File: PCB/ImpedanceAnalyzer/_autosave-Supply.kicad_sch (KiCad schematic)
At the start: 63 parts, among them U18 LM7812_TO220, U19 LM7912_TO220, U20 LM7806_TO220, U21 LT1086-3.3, U22 LM7805_TO220, U23 LM7905_TO220, U24 LM7906_TO220, U28 LD1117S25TR_SOT223

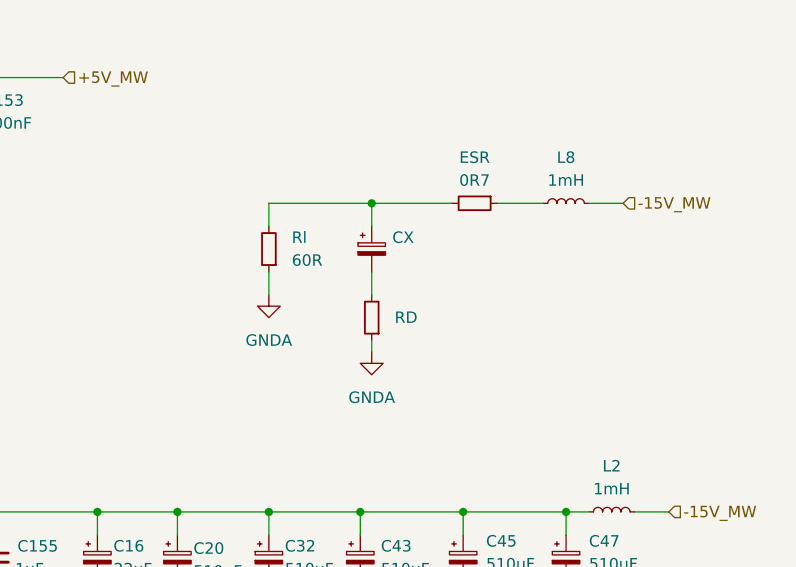
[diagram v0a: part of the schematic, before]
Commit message: docu doneski
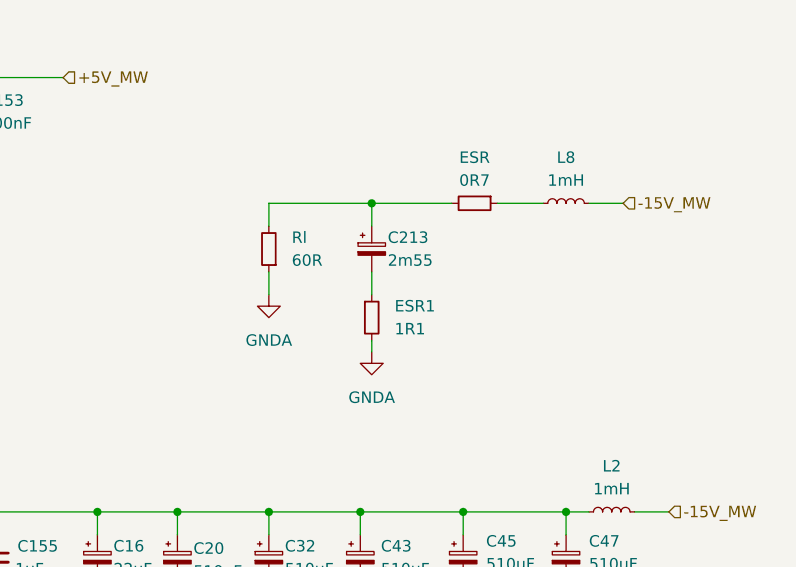
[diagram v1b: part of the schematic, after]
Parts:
- removed CX: CX, Capacitor_THT:CP_Radial_D10.0mm_P5.00mm, symbol Device:C_Polarized_Small
- removed R35: RD, Resistor_THT:R_Axial_DIN0207_L6.3mm_D2.5mm_P10.16mm_Horizontal, symbol Device:R_Small
- added C213: 2m55, Capacitor_THT:CP_Radial_D10.0mm_P5.00mm, symbol Device:C_Polarized_Small
- added ESR1: 1R1, Resistor_THT:R_Axial_DIN0207_L6.3mm_D2.5mm_P10.16mm_Horizontal, symbol Device:R_Small
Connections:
- net GNDA: now also ESR1.2
- net at ESR.2, Rl.2: now also C213.1
- new net: C213.2, ESR1.1
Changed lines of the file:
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@@
 	)
 	(symbol
+		(lib_id "Device:R_Small")
+		(at 228.6 104.14 0)
+		(unit 1)
+		(exclude_from_sim no)
+		(in_bom yes)
+		(on_board yes)
+		(dnp no)
+		(fields_autoplaced yes)
+		(property "Reference" "ESR1"
+			(at 231.14 102.8699 0)
+			(effects
+				(font
+					(size 1.27 1.27)
+				)
+				(justify left)
+			)
+		)
+		(property "Value" "1R1"
+			(at 231.14 105.4099 0)
+			(effects
+				(font
+					(size 1.27 1.27)
+				)
+				(justify left)
+			)
+		)
+		(property "Footprint" "Resistor_THT:R_Axial_DIN0207_L6.3mm_D2.5mm_P10.16mm_Horizontal"
+			(at 228.6 104.14 0)
+			(effects
+				(font
+					(size 1.27 1.27)
+				)
+				(hide yes)
+			)
+		)
+		(property "Datasheet" "~"
+			(at 228.6 104.14 0)
+			(effects
+				(font
+					(size 1.27 1.27)
+				)
+				(hide yes)
+			)
+		)
+		(property "Description" "Resistor, small symbol"
+			(at 228.6 104.14 0)
+			(effects
+				(font
+					(size 1.27 1.27)
+				)
+				(hide yes)
+			)
+		)
+		(pin "2"
+		)
+		(pin "1"
+		)
+		(instances
+			(project "ImpedanceAnalyzer"
+				(path "/08568624-f051-402a-adf3-1b03c2a769ee/bbce87d8-2d6b-4ada-9e87-44e06d8f0f46"
+					(reference "ESR1")
+					(unit 1)
+				)
+			)
+		)
+	)
+	(symbol
 		(lib_id "Device:LED_Small")
 		(at 35.56 160.02 270)
@@
 	(symbol
 		(lib_id "Device:C_Polarized_Small")
+		(at 228.6 96.52 0)
+		(unit 1)
+		(exclude_from_sim no)
+		(in_bom yes)
+		(on_board yes)
+		(dnp no)
+		(property "Reference" "C213"
+			(at 230.378 95.25 0)
+			(effects
+				(font
+					(size 1.27 1.27)
+				)
+				(justify left)
+			)
+		)
+		(property "Value" "2m55"
+			(at 230.378 97.79 0)
+			(effects
+				(font
+					(size 1.27 1.27)
+				)
+				(justify left)
+			)
+		)
+		(property "Footprint" "Capacitor_THT:CP_Radial_D10.0mm_P5.00mm"
+			(at 228.6 96.52 0)
+			(effects
+				(font
+					(size 1.27 1.27)
+				)
+				(hide yes)
+			)
+		)
+		(property "Datasheet" "~"
+			(at 228.6 96.52 0)
+			(effects
+				(font
+					(size 1.27 1.27)
+				)
+				(hide yes)
+			)
+		)
+		(property "Description" "Polarized capacitor, small symbol"
+			(at 228.6 96.52 0)
+			(effects
+				(font
+					(size 1.27 1.27)
+				)
+				(hide yes)
+			)
+		)
+		(pin "1"
+		)
+		(pin "2"
+		)
+		(instances
+			(project "ImpedanceAnalyzer"
+				(path "/08568624-f051-402a-adf3-1b03c2a769ee/bbce87d8-2d6b-4ada-9e87-44e06d8f0f46"
+					(reference "C213")
+					(unit 1)
+				)
+			)
+		)
+	)
+	(symbol
+		(lib_id "Device:C_Polarized_Small")
 		(at 198.12 30.48 0)
 		(unit 1)
@@
 	(symbol
 		(lib_id "Device:R_Small")
-		(at 228.6 104.14 180)
-		(unit 1)
-		(exclude_from_sim no)
-		(in_bom yes)
-		(on_board yes)
-		(dnp no)
-		(property "Reference" "R35"
-			(at 231.14 102.8699 0)
-			(effects
-				(font
-					(size 1.27 1.27)
-				)
-				(justify right)
-				(hide yes)
-			)
-		)
-		(property "Value" "RD"
-			(at 231.14 104.14 0)
-			(effects
-				(font
-					(size 1.27 1.27)
-				)
-				(justify right)
-			)
-		)
-		(property "Footprint" "Resistor_THT:R_Axial_DIN0207_L6.3mm_D2.5mm_P10.16mm_Horizontal"
-			(at 228.6 104.14 0)
-			(effects
-				(font
-					(size 1.27 1.27)
-				)
-				(hide yes)
-			)
-		)
-		(property "Datasheet" "~"
-			(at 228.6 104.14 0)
-			(effects
-				(font
-					(size 1.27 1.27)
-				)
-				(hide yes)
-			)
-		)
-		(property "Description" "Resistor, small symbol"
-			(at 228.6 104.14 0)
-			(effects
-				(font
-					(size 1.27 1.27)
-				)
-				(hide yes)
-			)
-		)
-		(pin "2"
-		)
-		(pin "1"
-		)
-		(instances
-			(project "ImpedanceAnalyzer"
-				(path "/08568624-f051-402a-adf3-1b03c2a769ee/bbce87d8-2d6b-4ada-9e87-44e06d8f0f46"
-					(reference "R35")
-					(unit 1)
-				)
-			)
-		)
-	)
-	(symbol
-		(lib_id "Device:R_Small")
 		(at 62.23 68.58 0)
 		(unit 1)
@@
 					(unit 1)
 				)
-			)
-		)
-	)
-	(symbol
-		(lib_id "Device:C_Polarized_Small")
-		(at 228.6 96.52 0)
-		(unit 1)
-		(exclude_from_sim no)
-		(in_bom yes)
-		(on_board yes)
-		(dnp no)
-		(property "Reference" "CX"
-			(at 230.886 95.25 0)
-			(effects
-				(font
-					(size 1.27 1.27)
-				)
-				(justify left)
-			)
-		)
-		(property "Value" "CX"
-			(at 230.886 97.79 0)
-			(effects
-				(font
-					(size 1.27 1.27)
-				)
-				(justify left)
-				(hide yes)
-			)
-		)
-		(property "Footprint" "Capacitor_THT:CP_Radial_D10.0mm_P5.00mm"
-			(at 228.6 96.52 0)
-			(effects
-				(font
-					(size 1.27 1.27)
-				)
-				(hide yes)
-			)
-		)
-		(property "Datasheet" "~"
-			(at 228.6 96.52 0)
-			(effects
-				(font
-					(size 1.27 1.27)
-				)
-				(hide yes)
-			)
-		)
-		(property "Description" "Polarized capacitor, small symbol"
-			(at 228.6 96.52 0)
-			(effects
-				(font
-					(size 1.27 1.27)
-				)
-				(hide yes)
-			)
-		)
-		(pin "1"
-		)
-		(pin "2"
-		)
-		(instances
-			(project "ImpedanceAnalyzer"
-				(path "/08568624-f051-402a-adf3-1b03c2a769ee/bbce87d8-2d6b-4ada-9e87-44e06d8f0f46"
-					(reference "CX")
-					(unit 1)
-				)
